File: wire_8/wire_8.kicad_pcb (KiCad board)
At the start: 2 copper layers, 18.8 x 13 mm, 2 parts, among them J1 Moat_Wire_8, J2 Moat_Wire_12

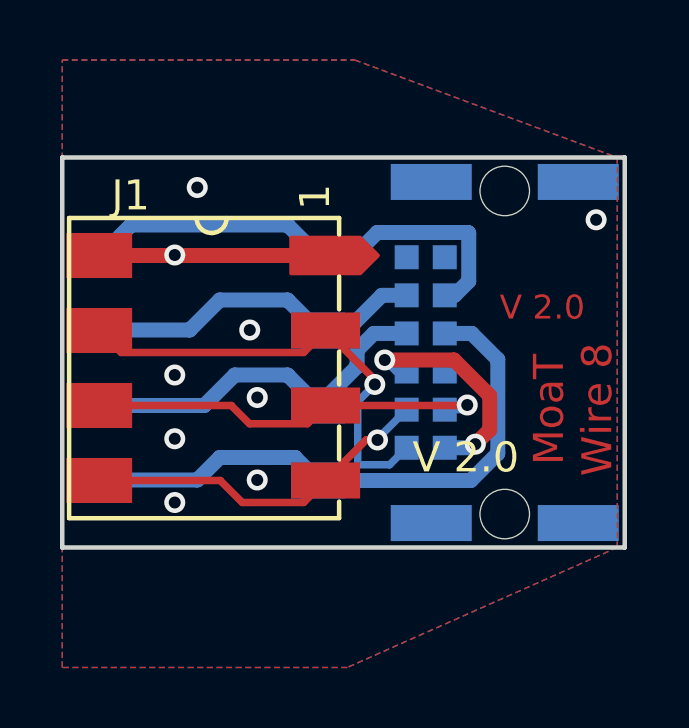
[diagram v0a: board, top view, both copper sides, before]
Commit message: No save for too long …
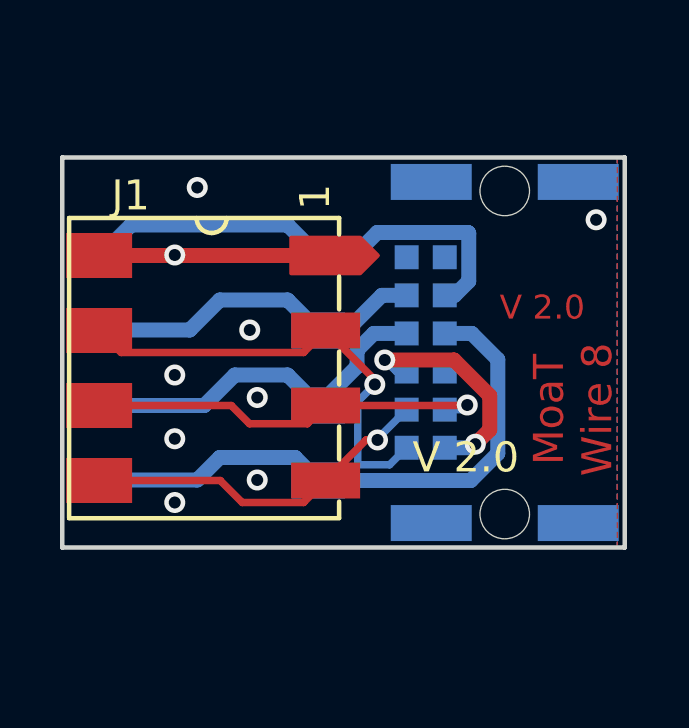
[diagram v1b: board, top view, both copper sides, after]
